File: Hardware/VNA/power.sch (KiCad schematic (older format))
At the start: 40 parts, among them Q1 RE1C002UN, U4 LP5912, U5 TVL755P, U6 MIC5366-1.8

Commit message: More schematic changes + updated functionals
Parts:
- removed U5: TVL755P, Package_DFN_QFN:DFN-6-1EP_2x2mm_P0.65mm_EP1x1.6mm, symbol VNA_Symbols:TVL755P
- added U5: LP5912, Package_DFN_QFN:DFN-6-1EP_2x2mm_P0.65mm_EP1x1.6mm, symbol VNA_Symbols:LP5912
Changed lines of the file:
@@
 	5150 3950 5150 3800
 Connection ~ 4950 3950
-Text Notes 4000 3550 0    100  ~ 0
+Text Notes 4000 3550 0    100  ~ 6
 1V8 LDO\n
 Wire Wire Line
@@
 	1    0    0    -1
 $EndComp
-Text Notes 1300 2150 0    100  ~ 0
+Text Notes 1300 2150 0    100  ~ 6
 5V (Filtered)
-Text HLabel 3350 3800 1    49   Input ~ 0
+Text HLabel 3350 3800 1    49   Input ~ 6
 3V3A
-Text HLabel 5150 3800 1    49   Input ~ 0
+Text HLabel 5150 3800 1    49   Input ~ 6
 1V8
-Text HLabel 2550 2400 1    49   Input ~ 0
+Text HLabel 2550 2400 1    49   Input ~ 6
 5V0
 Wire Wire Line
@@
 	1    0    0    -1
 $EndComp
-Text Notes 2250 3600 2    100  ~ 0
+Text Notes 2250 3600 2    100  ~ 6
 3V3A LDO
 Wire Wire Line
@@
 Wire Wire Line
 	2550 3950 2850 3950
-Text HLabel 2850 3850 1    49   Input ~ 0
+Text HLabel 2850 3850 1    49   Input ~ 6
 3V3A
 Connection ~ 2550 3950
@@
 $EndComp
 NoConn ~ 2150 4150
-$Comp
-L VNA_Symbols:TVL755P U5
-U 1 1 5CFCC1C6
-P 4200 2700
-F 0 "U5" H 4225 3125 50  0000 C CNN
-F 1 "TVL755P" H 4225 3034 50  0000 C CNN
-F 2 "Package_DFN_QFN:DFN-6-1EP_2x2mm_P0.65mm_EP1x1.6mm" H 4200 3150 100 0001 C CNN
-F 3 "" H 4200 3150 100 0001 C CNN
-	1    4200 2700
-	1    0    0    -1
-$EndComp
-Wire Wire Line
-	3750 2650 3750 2500
-Wire Wire Line
-	3750 2500 3900 2500
-Wire Wire Line
-	3750 2650 3900 2650
+Wire Wire Line
+	3750 2700 3750 2500
 $Comp
 L Device:C C32
@@
 Wire Wire Line
 	4950 2500 5250 2500
-Text HLabel 5250 2400 1    49   Input ~ 0
+Text HLabel 5250 2400 1    49   Input ~ 6
 3V3
 Connection ~ 4950 2500
@@
 $EndComp
 Wire Wire Line
-	4550 2650 4600 2650
-Wire Wire Line
-	4600 2650 4600 2750
-Wire Wire Line
-	4550 2950 4600 2950
-Connection ~ 4600 2950
-Wire Wire Line
-	4600 2950 4600 3050
-Wire Wire Line
-	4550 2850 4600 2850
-Connection ~ 4600 2850
-Wire Wire Line
-	4600 2850 4600 2950
-Wire Wire Line
-	4550 2750 4600 2750
-Connection ~ 4600 2750
-Wire Wire Line
-	4600 2750 4600 2850
+	4550 2700 4600 2700
+Wire Wire Line
+	4600 2700 4600 2800
+Wire Wire Line
+	4550 3000 4600 3000
+Connection ~ 4600 3000
+Wire Wire Line
+	4600 3000 4600 3100
+Wire Wire Line
+	4550 2900 4600 2900
+Connection ~ 4600 2900
+Wire Wire Line
+	4600 2900 4600 3000
+Wire Wire Line
+	4550 2800 4600 2800
+Connection ~ 4600 2800
+Wire Wire Line
+	4600 2800 4600 2900
 $Comp
 L power:GND #PWR037
 U 1 1 5CFD53FA
-P 4600 3050
-F 0 "#PWR037" H 4600 2800 50  0001 C CNN
-F 1 "GND" H 4605 2877 50  0000 C CNN
-F 2 "" H 4600 3050 50  0001 C CNN
-F 3 "" H 4600 3050 50  0001 C CNN
-	1    4600 3050
+P 4600 3100
+F 0 "#PWR037" H 4600 2850 50  0001 C CNN
+F 1 "GND" H 4605 2927 50  0000 C CNN
+F 2 "" H 4600 3100 50  0001 C CNN
+F 3 "" H 4600 3100 50  0001 C CNN
+	1    4600 3100
 	1    0    0    -1
 $EndComp
 Connection ~ 3750 2500
-Text Notes 4600 2200 2    100  ~ 0
+Text Notes 4600 2200 2    100  ~ 6
 3V3 LDO
 $Comp
@@
 	0    1    1    0
 $EndComp
-Text HLabel 1250 1400 0    49   Input ~ 0
+Text HLabel 1250 1400 0    49   Input ~ 6
 VBUS
 Wire Wire Line
 	1900 1400 2200 1400
-Text Label 2300 1400 0    50   ~ 0
+Text Label 2300 1400 0    50   ~ 6
 VIN
-Text Label 1050 2400 1    50   ~ 0
+Text Label 1050 2400 1    50   ~ 6
 VIN
-Text Label 3350 2400 1    50   ~ 0
+Text Label 3350 2400 1    50   ~ 6
 VIN
-Text Label 1100 3850 1    50   ~ 0
+Text Label 1100 3850 1    50   ~ 6
 VIN
-Text Notes 1200 1150 0    100  ~ 0
+Text Notes 1200 1150 0    100  ~ 6
 Input Protection
 Wire Wire Line
@@
 Wire Wire Line
 	6600 2600 6600 2550
-Text HLabel 6600 2550 1    50   Input ~ 0
+Text HLabel 6600 2550 1    50   Input ~ 6
 3V3A
-Text HLabel 6150 3500 0    50   Input ~ 0
+Text HLabel 6150 3500 0    50   Input ~ 6
 1V8
 Wire Wire Line
@@
 	1    0    0    -1
 $EndComp
-Text Notes 6800 2200 0    100  ~ 0
+Text Notes 6800 2200 0    100  ~ 6
 Voltage Rail LEDs
 Wire Wire Line
 	7250 2600 7250 2550
-Text HLabel 7250 2550 1    50   Input ~ 0
+Text HLabel 7250 2550 1    50   Input ~ 6
 3V3A
 Wire Wire Line
@@
 Wire Wire Line
 	7650 2600 7650 2550
-Text HLabel 7650 2550 1    50   Input ~ 0
+Text HLabel 7650 2550 1    50   Input ~ 6
 3V3
 Wire Wire Line
@@
 Wire Wire Line
 	8050 2600 8050 2550
-Text HLabel 8050 2550 1    50   Input ~ 0
+Text HLabel 8050 2550 1    50   Input ~ 6
 5V0
 Wire Wire Line
@@
 	1    0    0    -1
 $EndComp
-Text HLabel 8400 2550 1    49   Input ~ 0
+Text HLabel 8400 2550 1    49   Input ~ 6
 VBUS
 Connection ~ 5150 3950
@@
 	1    0    0    -1
 $EndComp
-Text Notes 9150 2200 0    100  ~ 0
+Text Notes 9150 2200 0    100  ~ 6
 Ground Test Points
 $Comp
@@
 	0    1    1    0
 $EndComp
+$Comp
+L VNA_Symbols:LP5912 U5
+U 1 1 5CAEAD8A
+P 4250 2750
+F 0 "U5" H 4100 3200 49  0000 C CNN
+F 1 "LP5912" H 4200 3100 49  0000 C CNN
+F 2 "Package_DFN_QFN:DFN-6-1EP_2x2mm_P0.65mm_EP1x1.6mm" H 4200 3100 49  0001 C CNN
+F 3 "" H 4200 3100 49  0001 C CNN
+	1    4250 2750
+	1    0    0    -1
+$EndComp
+Wire Wire Line
+	3750 2700 3950 2700
+Wire Wire Line
+	3750 2500 3950 2500
 $EndSCHEMATC

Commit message: first day of layout / routing done
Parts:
- F1: footprint VNA_Footprints:Fuse_1206_3216Metric -> VNA_Footprints:Fuse_0805_2012Metric
- Q1: footprint Package_TO_SOT_SMD:SOT-89-3 -> Package_TO_SOT_SMD:SOT-416
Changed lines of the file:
@@
 	5150 3950 5150 3800
 Connection ~ 4950 3950
-Text Notes 4000 3550 0    100  ~ 6
+Text Notes 4000 3550 0    100  ~ 20
 1V8 LDO\n
 Wire Wire Line
@@
 	1    0    0    -1
 $EndComp
-Text Notes 1300 2150 0    100  ~ 6
+Text Notes 1300 2150 0    100  ~ 20
 5V (Filtered)
-Text HLabel 3350 3800 1    49   Input ~ 6
+Text HLabel 3350 3800 1    49   Input ~ 10
 3V3A
-Text HLabel 5150 3800 1    49   Input ~ 6
+Text HLabel 5150 3800 1    49   Input ~ 10
 1V8
-Text HLabel 2550 2400 1    49   Input ~ 6
+Text HLabel 2550 2400 1    49   Input ~ 10
 5V0
 Wire Wire Line
@@
 	1    0    0    -1
 $EndComp
-Text Notes 2250 3600 2    100  ~ 6
+Text Notes 2250 3600 2    100  ~ 20
 3V3A LDO
 Wire Wire Line
@@
 Wire Wire Line
 	2550 3950 2850 3950
-Text HLabel 2850 3850 1    49   Input ~ 6
+Text HLabel 2850 3850 1    49   Input ~ 10
 3V3A
 Connection ~ 2550 3950
@@
 Wire Wire Line
 	4950 2500 5250 2500
-Text HLabel 5250 2400 1    49   Input ~ 6
+Text HLabel 5250 2400 1    49   Input ~ 10
 3V3
 Connection ~ 4950 2500
@@
 $EndComp
 Connection ~ 3750 2500
-Text Notes 4600 2200 2    100  ~ 6
+Text Notes 4600 2200 2    100  ~ 20
 3V3 LDO
 $Comp
@@
 F 0 "F1" V 1700 1400 50  0000 C CNN
 F 1 "500mA Polyfuse" V 1900 1400 50  0000 C CNN
-F 2 "VNA_Footprints:Fuse_1206_3216Metric" H 1850 1200 50  0001 L CNN
+F 2 "VNA_Footprints:Fuse_0805_2012Metric" H 1850 1200 50  0001 L CNN
 F 3 "~" H 1800 1400 50  0001 C CNN
 	1    1800 1400
 	0    1    1    0
 $EndComp
-Text HLabel 1250 1400 0    49   Input ~ 6
+Text HLabel 1250 1400 0    49   Input ~ 10
 VBUS
 Wire Wire Line
 	1900 1400 2200 1400
-Text Label 2300 1400 0    50   ~ 6
+Text Label 2300 1400 0    50   ~ 10
 VIN
-Text Label 1050 2400 1    50   ~ 6
+Text Label 1050 2400 1    50   ~ 10
 VIN
-Text Label 3350 2400 1    50   ~ 6
+Text Label 3350 2400 1    50   ~ 10
 VIN
-Text Label 1100 3850 1    50   ~ 6
+Text Label 1100 3850 1    50   ~ 10
 VIN
-Text Notes 1200 1150 0    100  ~ 6
+Text Notes 1200 1150 0    100  ~ 20
 Input Protection
 Wire Wire Line
@@
 F 0 "Q1" H 6706 3546 50  0000 L CNN
 F 1 "RE1C002UN" H 6706 3455 50  0000 L CNN
-F 2 "Package_TO_SOT_SMD:SOT-89-3" H 6700 3600 50  0001 C CNN
+F 2 "Package_TO_SOT_SMD:SOT-416" H 6700 3600 50  0001 C CNN
 F 3 "~" H 6500 3500 50  0001 C CNN
 	1    6500 3500
@@
 Wire Wire Line
 	6600 2600 6600 2550
-Text HLabel 6600 2550 1    50   Input ~ 6
+Text HLabel 6600 2550 1    50   Input ~ 10
 3V3A
-Text HLabel 6150 3500 0    50   Input ~ 6
+Text HLabel 6150 3500 0    50   Input ~ 10
 1V8
 Wire Wire Line
@@
 	1    0    0    -1
 $EndComp
-Text Notes 6800 2200 0    100  ~ 6
+Text Notes 6800 2200 0    100  ~ 20
 Voltage Rail LEDs
 Wire Wire Line
 	7250 2600 7250 2550
-Text HLabel 7250 2550 1    50   Input ~ 6
+Text HLabel 7250 2550 1    50   Input ~ 10
 3V3A
 Wire Wire Line
@@
 Wire Wire Line
 	7650 2600 7650 2550
-Text HLabel 7650 2550 1    50   Input ~ 6
+Text HLabel 7650 2550 1    50   Input ~ 10
 3V3
 Wire Wire Line
@@
 Wire Wire Line
 	8050 2600 8050 2550
-Text HLabel 8050 2550 1    50   Input ~ 6
+Text HLabel 8050 2550 1    50   Input ~ 10
 5V0
 Wire Wire Line
@@
 	1    0    0    -1
 $EndComp
-Text HLabel 8400 2550 1    49   Input ~ 6
+Text HLabel 8400 2550 1    49   Input ~ 10
 VBUS
 Connection ~ 5150 3950
@@
 	1    0    0    -1
 $EndComp
-Text Notes 9150 2200 0    100  ~ 6
+Text Notes 9150 2200 0    100  ~ 20
 Ground Test Points
 $Comp

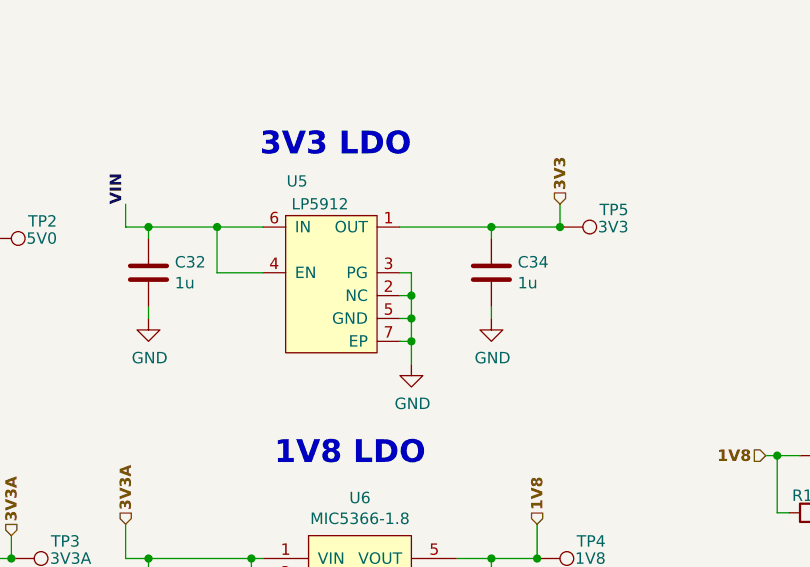
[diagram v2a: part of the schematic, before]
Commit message: no unrouted nets!
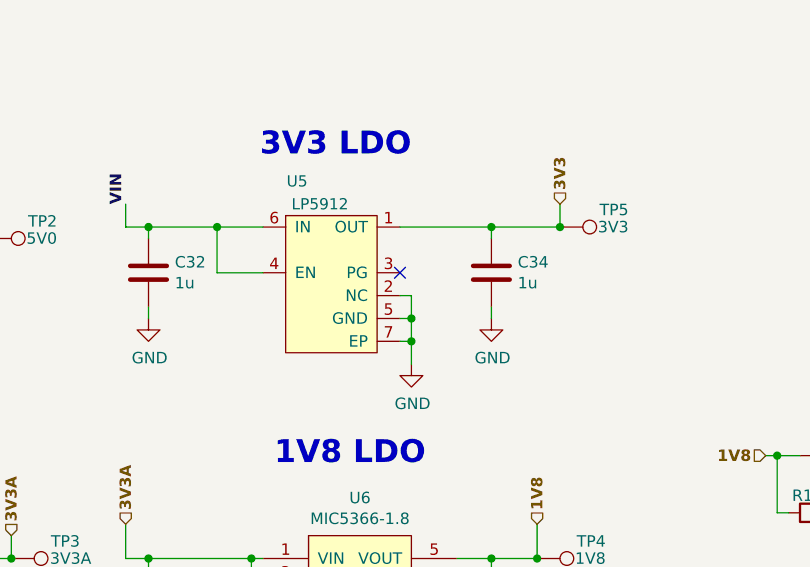
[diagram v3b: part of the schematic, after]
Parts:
- Q1: footprint Package_TO_SOT_SMD:SOT-416 -> VNA_Footprints:SOT-416
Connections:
- net GND: no longer U5.3 (PG)
- no-connect marks 1 -> 2
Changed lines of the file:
@@
 $EndComp
-Wire Wire Line
-	4550 2700 4600 2700
-Wire Wire Line
-	4600 2700 4600 2800
 Wire Wire Line
 	4550 3000 4600 3000
@@
 Wire Wire Line
 	4550 2800 4600 2800
-Connection ~ 4600 2800
 Wire Wire Line
 	4600 2800 4600 2900
@@
 F 0 "Q1" H 6706 3546 50  0000 L CNN
 F 1 "RE1C002UN" H 6706 3455 50  0000 L CNN
-F 2 "Package_TO_SOT_SMD:SOT-416" H 6700 3600 50  0001 C CNN
+F 2 "VNA_Footprints:SOT-416" H 6700 3600 50  0001 C CNN
 F 3 "~" H 6500 3500 50  0001 C CNN
 	1    6500 3500
@@
 Wire Wire Line
 	3750 2500 3950 2500
+NoConn ~ 4550 2700
 $EndSCHEMATC
